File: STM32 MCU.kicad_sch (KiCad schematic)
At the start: 33 parts, among them SW3 SW_Push, SW4 SW_Push, U2 STM32G474RETx, U4 RV-3028-C7, Y1 Crystal, Y3 Crystal

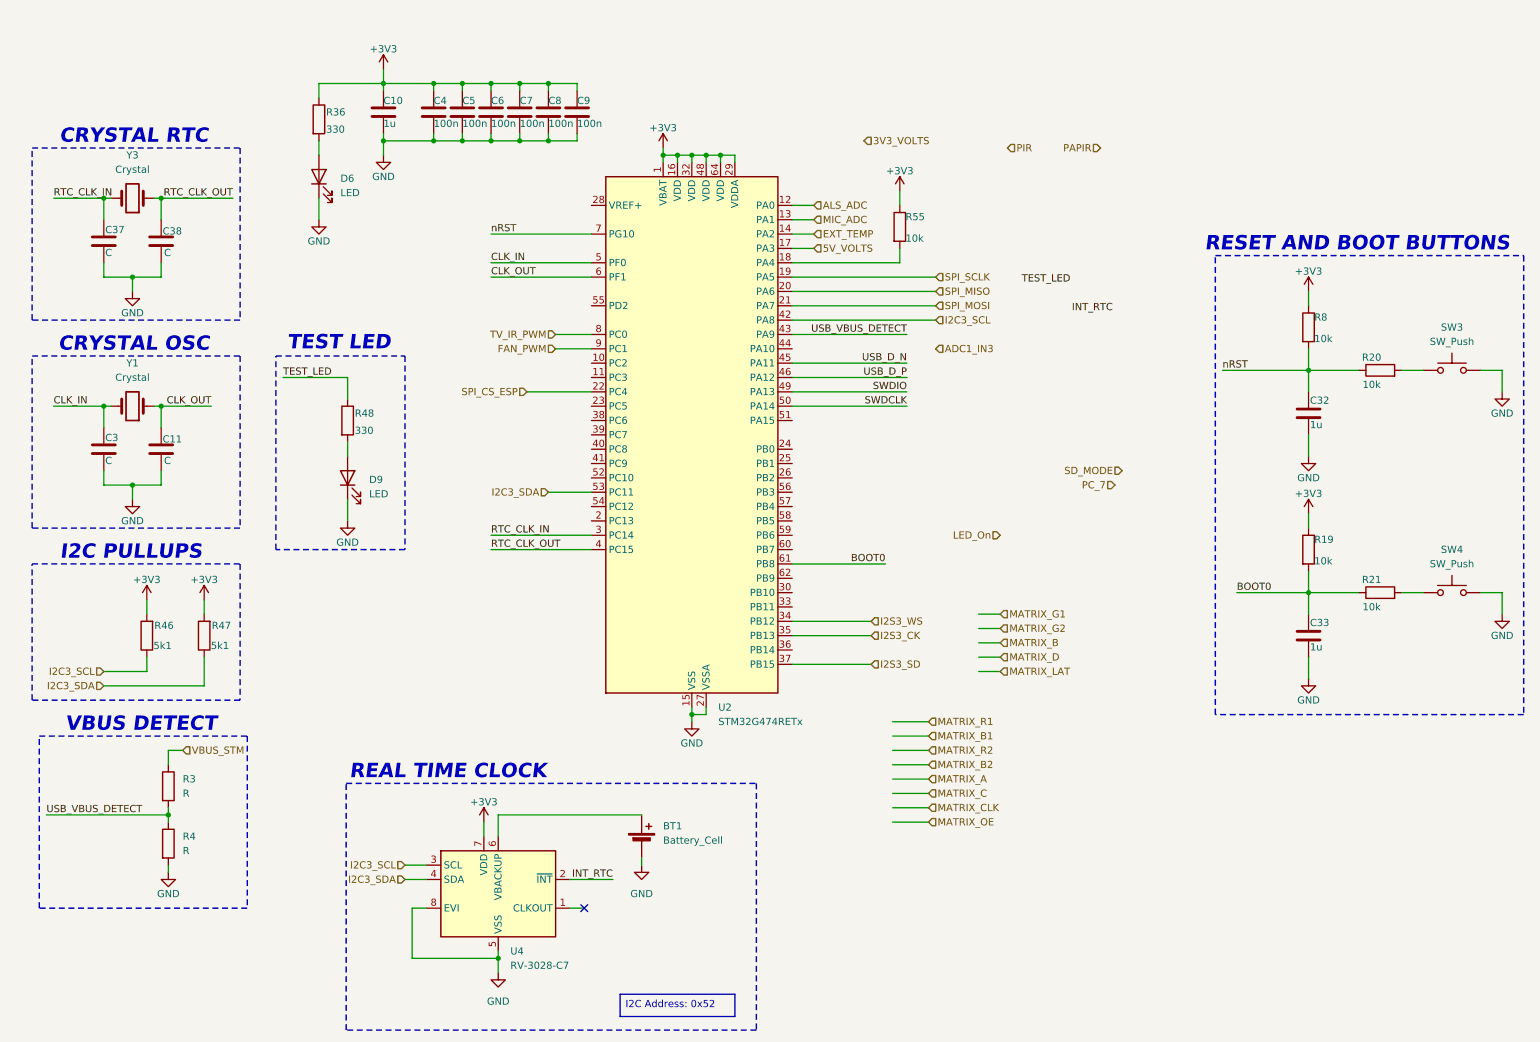
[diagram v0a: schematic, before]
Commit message: STM32 Work
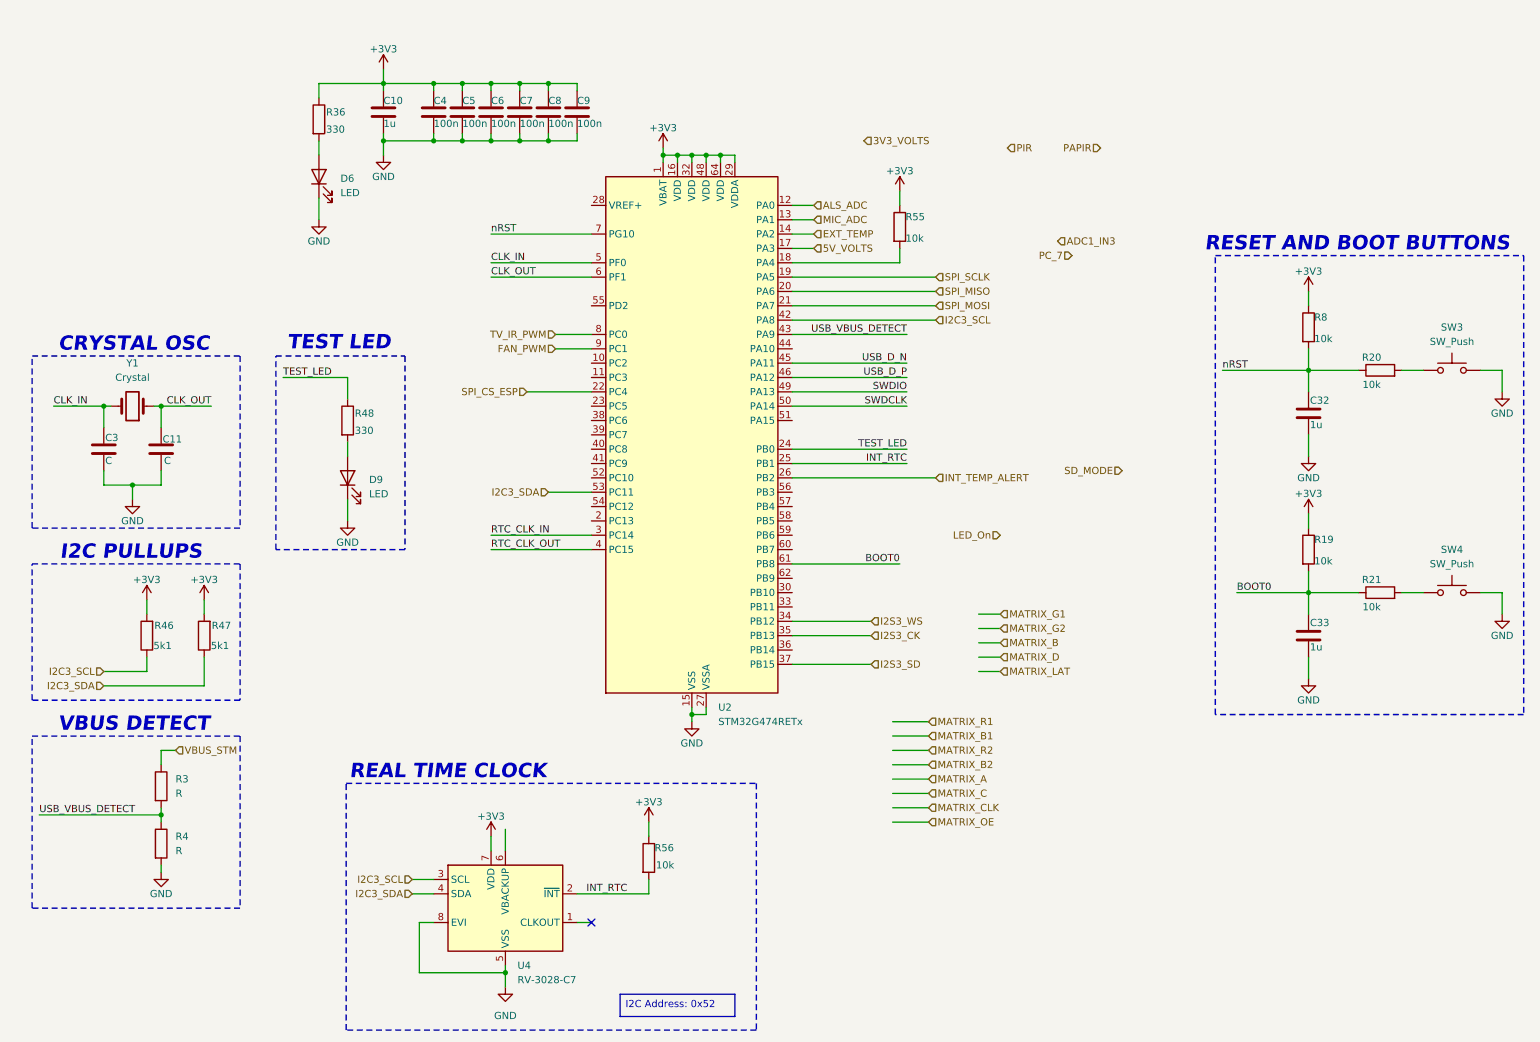
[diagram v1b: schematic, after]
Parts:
- removed BT1: Battery_Cell, Battery:BatteryHolder_Keystone_3000_1x12mm, symbol Device:Battery_Cell
- removed C37, C38: C, symbol Device:C
- removed Y3: Crystal, Package_QFP:LQFP-64_10x10mm_P0.5mm, symbol Device:Crystal
- added R56: 10k, Package_DIP:DIP-8_W7.62mm, symbol Device:R
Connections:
- net +3V3: now also R56.1
- net INT_RTC: now also U2.25 (PB1), R56.2
- net TEST_LED: now also U2.24 (PB0)
- net INT_TEMP_ALERT: now reaches U2.26 (PB2)
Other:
- note removed: "CRYSTAL RTC"
- moved on the sheet: R3, R4, U4

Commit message: Revert "Merge branch 'main' of https://github.com/pequeno212/PCB_SeniorDesign_team20"
This reverts commit 8ddd870afa6ea88a1f78691f7845b0b29e49b9ae, reversing
changes made to b7b9844e80cb26773f88e7278ccd95378529a98d.
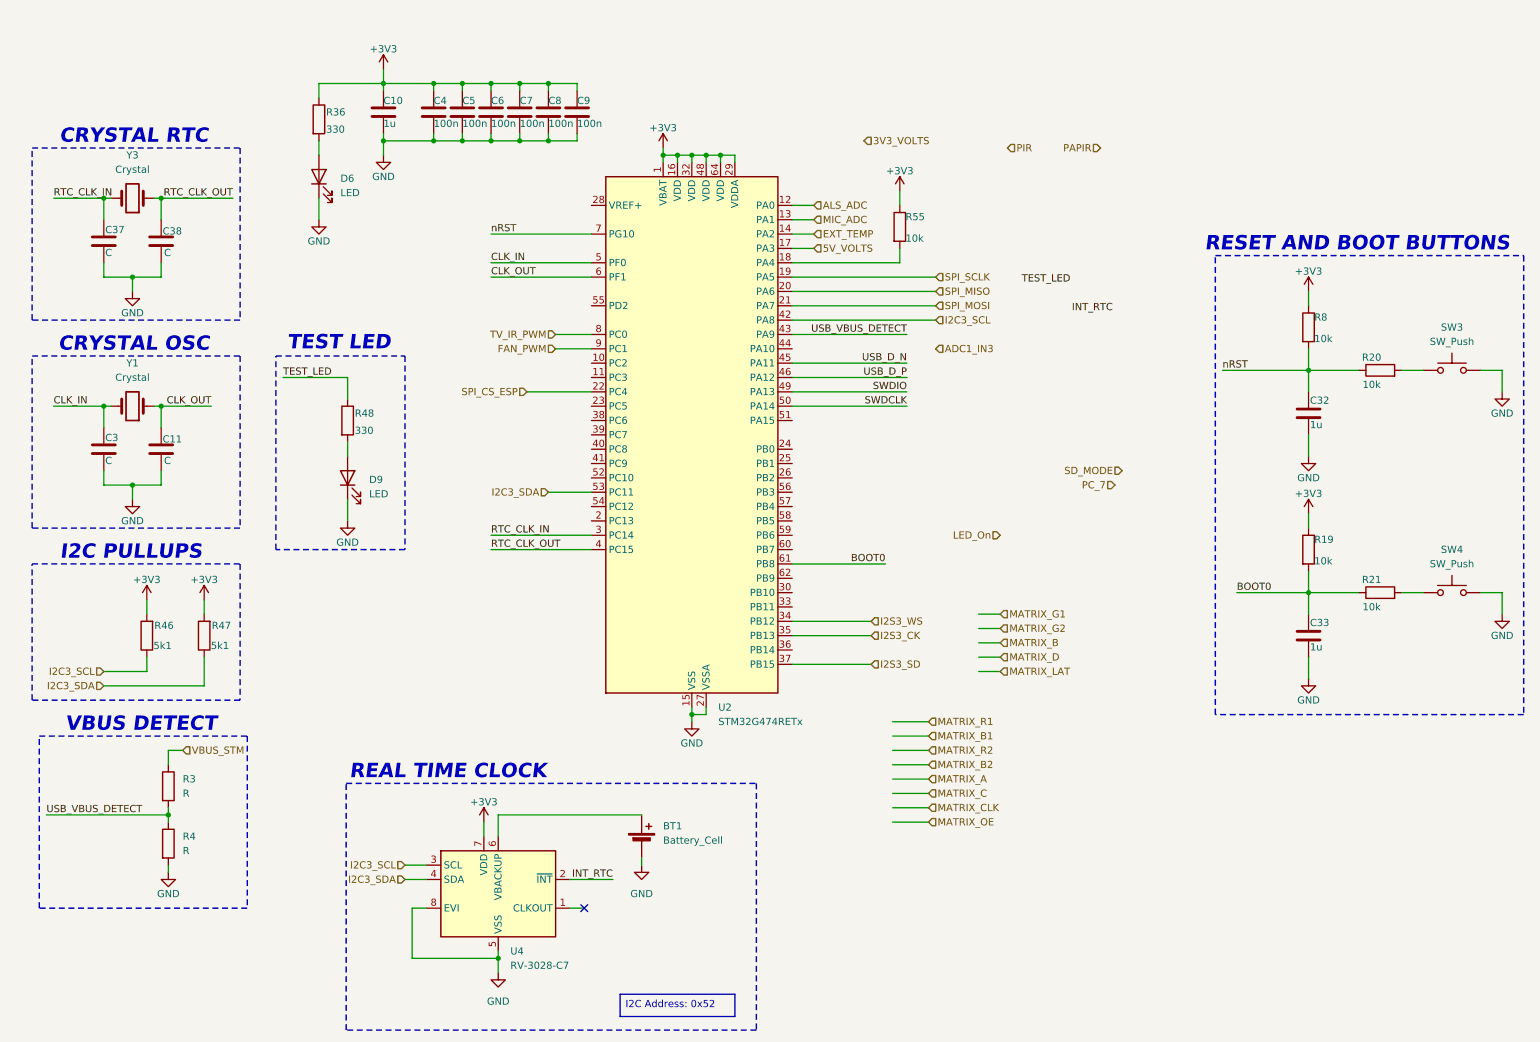
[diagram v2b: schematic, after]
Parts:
- removed R56: 10k, Package_DIP:DIP-8_W7.62mm, symbol Device:R
- added BT1: Battery_Cell, Battery:BatteryHolder_Keystone_3000_1x12mm, symbol Device:Battery_Cell
- added C37, C38: C, symbol Device:C
- added Y3: Crystal, Package_QFP:LQFP-64_10x10mm_P0.5mm, symbol Device:Crystal
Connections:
- net GND: now also BT1.2 (-), C37.2, C38.2
- net INT_RTC: no longer U2.25 (PB1)
- net RTC_CLK_IN: now also C37.1, Y3.2
- net RTC_CLK_OUT: now also C38.1, Y3.1
- net TEST_LED: no longer U2.24 (PB0)
- net at U4.6 (VBACKUP): now also BT1.1 (+)
- net INT_TEMP_ALERT: no longer names the net of U2.26 (PB2)
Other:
- note added: "CRYSTAL RTC"
- moved on the sheet: R3, R4, U4

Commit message: Major Changes - Schematic Done??
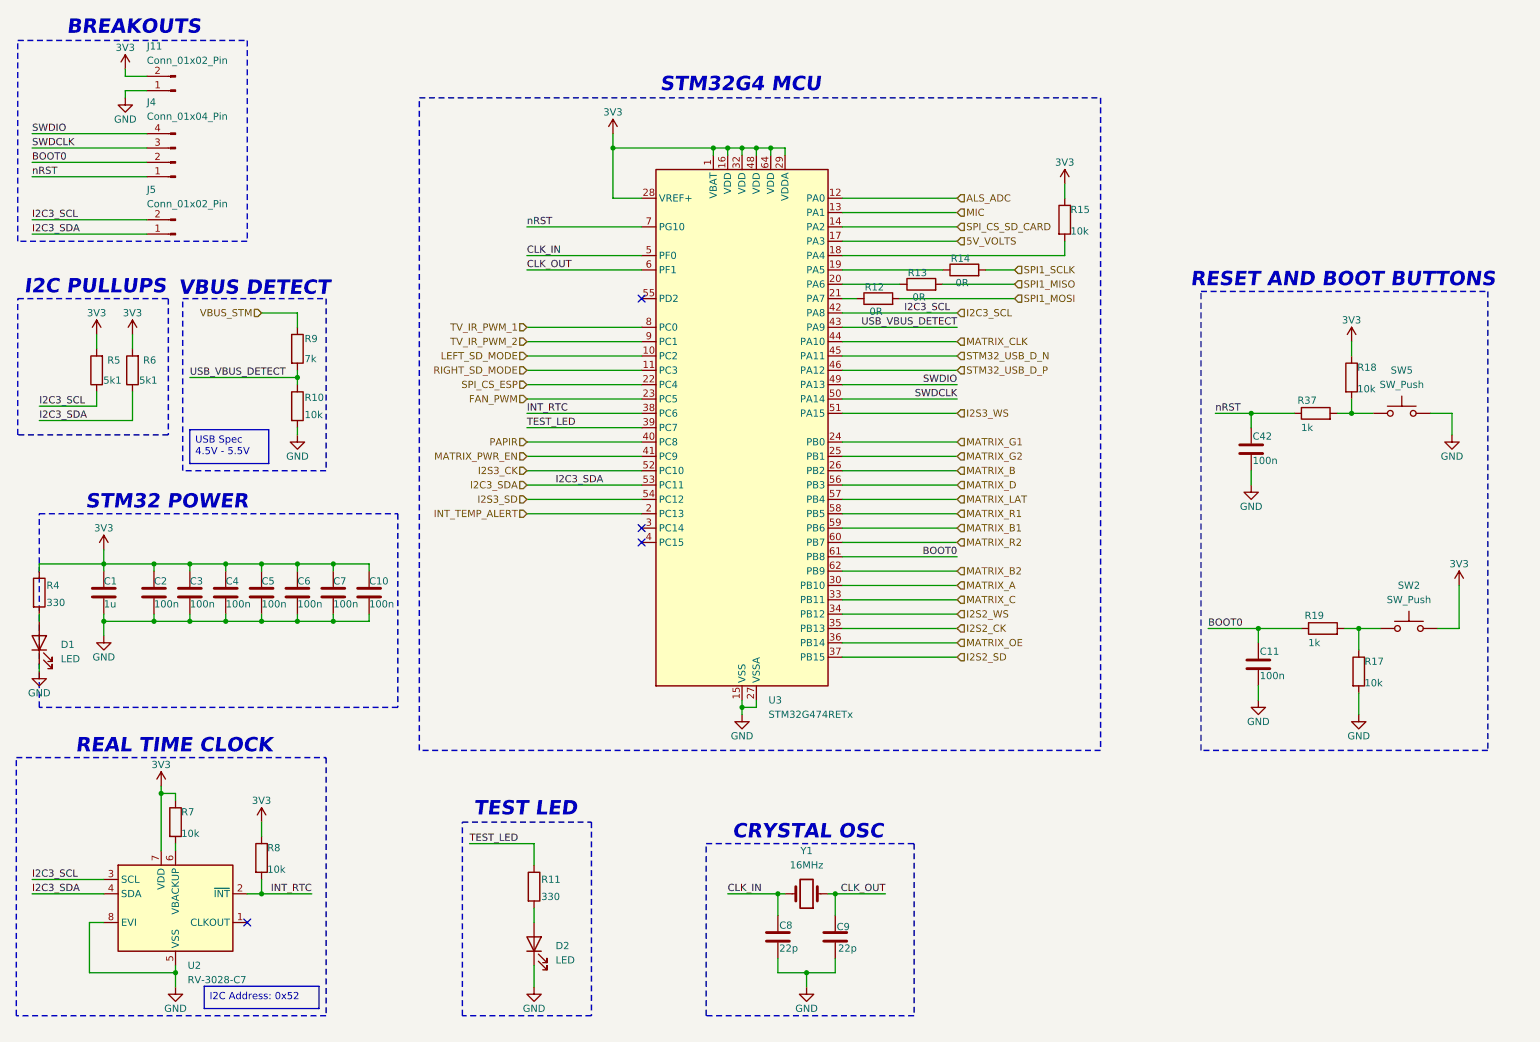
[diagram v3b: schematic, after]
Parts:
- removed BT1: Battery_Cell, Battery:BatteryHolder_Keystone_3000_1x12mm, symbol Device:Battery_Cell
- removed C32: 1u, symbol Device:C
- removed C37, C38: C, symbol Device:C
- removed R20: 10k, Package_DIP:DIP-8_W7.62mm, symbol Device:R
- removed SW3: SW_Push, Package_DIP:DIP-8_W7.62mm, symbol Switch:SW_Push
- removed Y3: Crystal, Package_QFP:LQFP-64_10x10mm_P0.5mm, symbol Device:Crystal
- added C10, C42: 100n, Capacitor_SMD:C_0603_1608Metric, symbol Device:C
- added J11, J5: Conn_01x02_Pin, Connector_PinHeader_2.54mm:PinHeader_1x02_P2.54mm_Vertical, symbol Connector:Conn_01x02_Pin
- added J4: Conn_01x04_Pin, Connector_PinHeader_2.54mm:PinHeader_1x04_P2.54mm_Vertical, symbol Connector:Conn_01x04_Pin
- added R12, R13, R14: 0R, Resistor_SMD:R_0603_1608Metric, symbol Device:R
- added R18, R7: 10k, Resistor_SMD:R_0603_1608Metric, symbol Device:R
- added R37: 1k, Resistor_SMD:R_0603_1608Metric, symbol Device:R
- added SW5: SW_Push, Button_Switch_THT:SW_PUSH_6mm, symbol Switch:SW_Push
- C1: renamed from C10; footprint (none) -> Capacitor_SMD:C_0603_1608Metric
- C11: renamed from C33; value 1u -> 100n; footprint (none) -> Capacitor_SMD:C_0603_1608Metric
- C2: renamed from C4; footprint (none) -> Capacitor_SMD:C_0603_1608Metric
- C3: renamed from C5; footprint (none) -> Capacitor_SMD:C_0603_1608Metric
- C4: renamed from C6; footprint (none) -> Capacitor_SMD:C_0603_1608Metric
- C5: renamed from C7; footprint (none) -> Capacitor_SMD:C_0603_1608Metric
- C6: renamed from C8; footprint (none) -> Capacitor_SMD:C_0603_1608Metric
- C7: renamed from C9; footprint (none) -> Capacitor_SMD:C_0603_1608Metric
- C8: renamed from C3; value C -> 22p; footprint (none) -> Capacitor_SMD:C_0603_1608Metric
- C9: renamed from C11; value C -> 22p; footprint (none) -> Capacitor_SMD:C_0603_1608Metric
- D1: renamed from D6; footprint (none) -> LED_SMD:LED_0603_1608Metric
- D2: renamed from D9; footprint (none) -> LED_SMD:LED_0603_1608Metric
- R10: renamed from R4; value R -> 10k; footprint Package_DIP:DIP-8_W7.62mm -> Resistor_SMD:R_0603_1608Metric
- R11: renamed from R48; footprint Package_DIP:DIP-8_W7.62mm -> Resistor_SMD:R_0603_1608Metric
- R15: renamed from R55; footprint Package_DIP:DIP-8_W7.62mm -> Resistor_SMD:R_0603_1608Metric
- R17: renamed from R19; footprint Package_DIP:DIP-8_W7.62mm -> Resistor_SMD:R_0603_1608Metric
- R19: renamed from R21; value 10k -> 1k; footprint Package_DIP:DIP-8_W7.62mm -> Resistor_SMD:R_0603_1608Metric
- R4: renamed from R36; footprint Package_DIP:DIP-8_W7.62mm -> Resistor_SMD:R_0603_1608Metric
- R5: renamed from R46; footprint Package_DIP:DIP-8_W7.62mm -> Resistor_SMD:R_0603_1608Metric
- R6: renamed from R47; footprint Package_DIP:DIP-8_W7.62mm -> Resistor_SMD:R_0603_1608Metric
- R8: footprint Package_DIP:DIP-8_W7.62mm -> Resistor_SMD:R_0603_1608Metric
- R9: renamed from R3; value R -> 7k; footprint Package_DIP:DIP-8_W7.62mm -> Resistor_SMD:R_0603_1608Metric
- SW2: renamed from SW4; footprint Package_DIP:DIP-8_W7.62mm -> Button_Switch_THT:SW_PUSH_6mm
- Y1: value Crystal -> 16MHz; footprint Package_QFP:LQFP-64_10x10mm_P0.5mm -> Crystal:Crystal_SMD_ECS_CSM3X-2Pin_7.6x4.1mm
- renumbered U4 to U2, U2 to U3
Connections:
- net BOOT0: now also J4.2 (Pin_2); no longer R17.2
- net FAN_PWM: now also U3.23 (PC5); no longer U3.9 (PC1)
- net GND: now also R17.2, C10.2, C42.2, J11.1 (Pin_1), SW5.2; no longer SW2.2
- net I2C3_SCL: now also J5.2 (Pin_2)
- net I2C3_SDA: now also J5.1 (Pin_1)
- net I2S3_CK: now also U3.52 (PC10); no longer U3.35 (PB13)
- net I2S3_SD: now also U3.54 (PC12); no longer U3.37 (PB15)
- net I2S3_WS: now also U3.51 (PA15); no longer U3.34 (PB12)
- net INT_RTC: now also R8.2, U3.38 (PC6)
- net MATRIX_A: now also U3.30 (PB10)
- net MATRIX_B: now also U3.26 (PB2)
- net MATRIX_B1: now also U3.59 (PB6)
- net MATRIX_B2: now also U3.62 (PB9)
- net MATRIX_C: now also U3.33 (PB11)
- net MATRIX_CLK: now also U3.44 (PA10)
- net MATRIX_D: now also U3.56 (PB3)
- net MATRIX_G1: now also U3.24 (PB0)
- net MATRIX_G2: now also U3.25 (PB1)
- net MATRIX_LAT: now also U3.57 (PB4)
- net MATRIX_OE: now also U3.36 (PB14)
- net MATRIX_R1: now also U3.58 (PB5)
- net MATRIX_R2: now also U3.60 (PB7)
- net PAPIR: now also U3.40 (PC8)
- net SWDCLK: now also J4.3 (Pin_3)
- net SWDIO: now also J4.4 (Pin_4)
- net TEST_LED: now also U3.39 (PC7)
- net nRST: now also C42.1, J4.1 (Pin_1), R37.1; no longer R8.2
- net at R19.2, SW2.1: now also R17.1
- net at U2.6 (VBACKUP): now also R7.2
- net LEFT_SD_MODE: now reaches U3.10 (PC2)
- net RIGHT_SD_MODE: now reaches U3.11 (PC3)
- net INT_TEMP_ALERT: now reaches U3.2 (PC13)
- net 3V3: now reaches U3.28 (VREF+)
- net 3V3: now also C1.1, C2.1, C3.1, C4.1, C5.1, C6.1, C7.1, R15.1, R4.1, R5.2, R6.2, R8.1, SW2.2, U2.7 (VDD), U3.1 (VBAT), U3.16 (VDD), U3.29 (VDDA), U3.32 (VDD), U3.48 (VDD), U3.64 (VDD), C10.1, J11.2 (Pin_2), R18.1, R7.1
- net MATRIX_PWR_EN: now reaches U3.41 (PC9)
- removed net +3V3: C1.1, C2.1, C3.1, C4.1, C5.1, C6.1, C7.1, R15.1, R17.1, R4.1, R5.2, R6.2, R8.1, U2.7 (VDD), U3.1 (VBAT), U3.16 (VDD), U3.29 (VDDA), U3.32 (VDD), U3.48 (VDD), U3.64 (VDD)
- net EXT_TEMP renamed SPI_CS_SD_CARD
- net MIC_ADC renamed MIC
- net RTC_CLK_IN: no longer names the net of U3.3 (PC14)
- net RTC_CLK_OUT: no longer names the net of U3.4 (PC15)
- net SPI_MISO: no longer names the net of U3.20 (PA6)
- net SPI_MISO: now also R13.1
- net SPI_MOSI: no longer names the net of U3.21 (PA7)
- net SPI_MOSI: now also R12.1
- net SPI_SCLK: no longer names the net of U3.19 (PA5)
- net SPI_SCLK: now also R14.1
- net TV_IR_PWM renamed TV_IR_PWM_1
- net USB_D_N renamed STM32_USB_D_N
- net USB_D_P renamed STM32_USB_D_P
- new net: R18.2, R37.2, SW5.1
- new net I2S2_CK: U3.35 (PB13)
- new net I2S2_SD: U3.37 (PB15)
- new net I2S2_WS: U3.34 (PB12)
- new net SPI1_MISO: R13.2
- new net SPI1_MOSI: R12.2
- new net SPI1_SCLK: R14.2
- new net TV_IR_PWM_2: U3.9 (PC1)
- no-connect marks 1 -> 4
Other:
- note added: "BREAKOUTS"
- note added: "STM32 POWER"
- note added: "STM32G4 MCU"
- note removed: "CRYSTAL RTC"
- moved on the sheet: C1, C11, C2, C3, C4, C5, C6, C7, C8, C9, D1, D2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
